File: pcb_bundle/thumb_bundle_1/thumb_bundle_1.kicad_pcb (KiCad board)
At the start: 2 copper layers, 100.6 x 101.6 mm, 55 parts

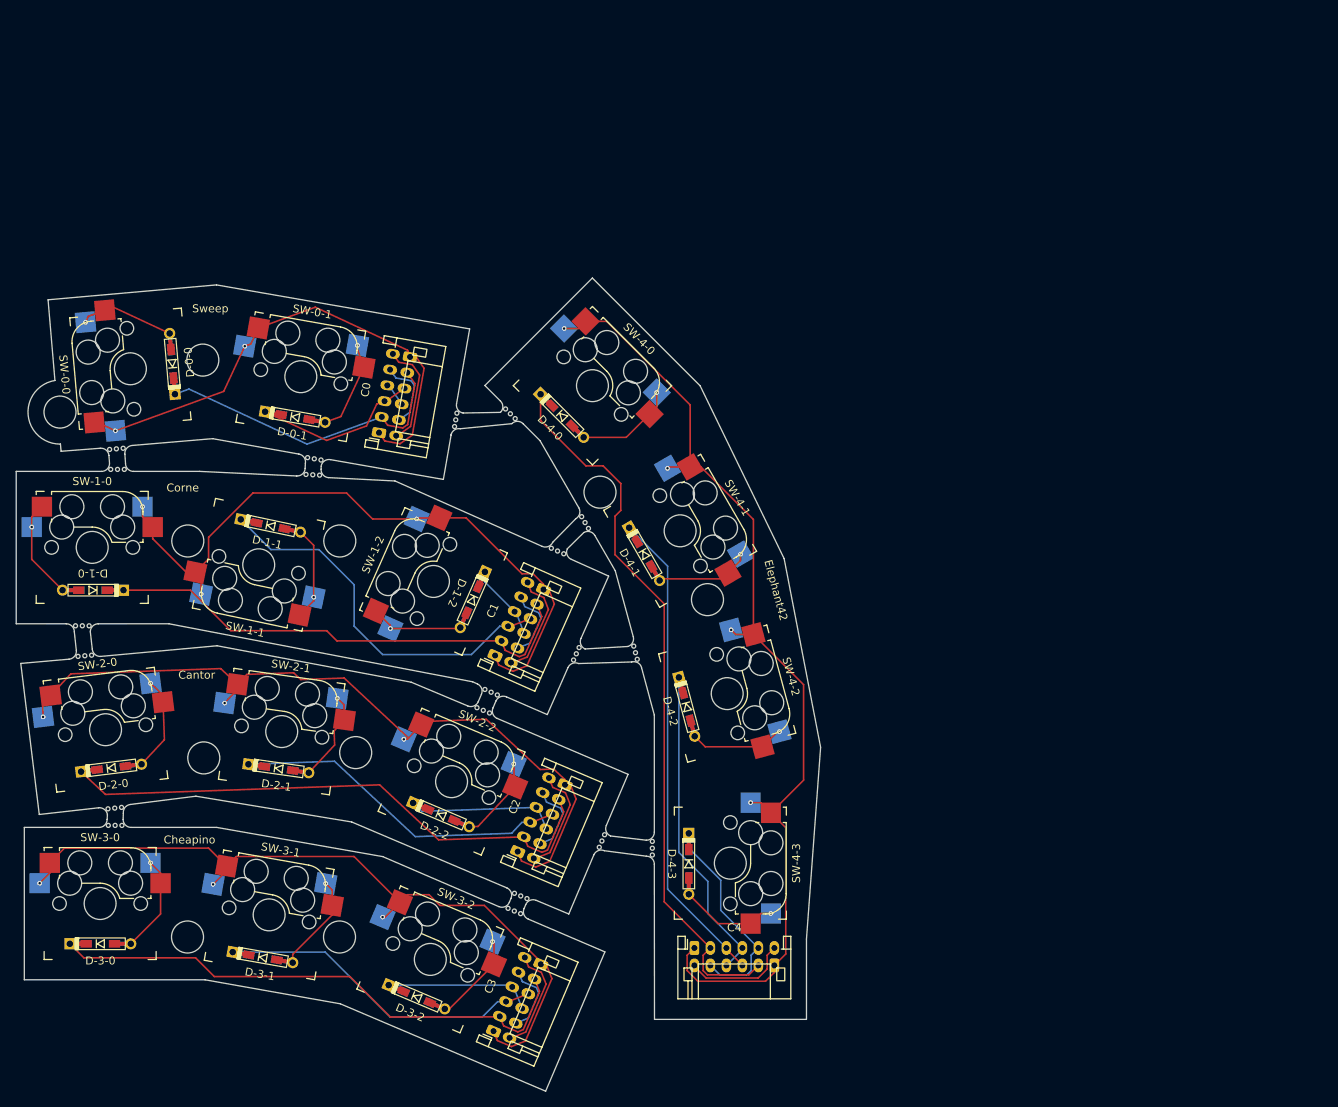
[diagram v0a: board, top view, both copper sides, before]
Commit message: [unstable] interim state
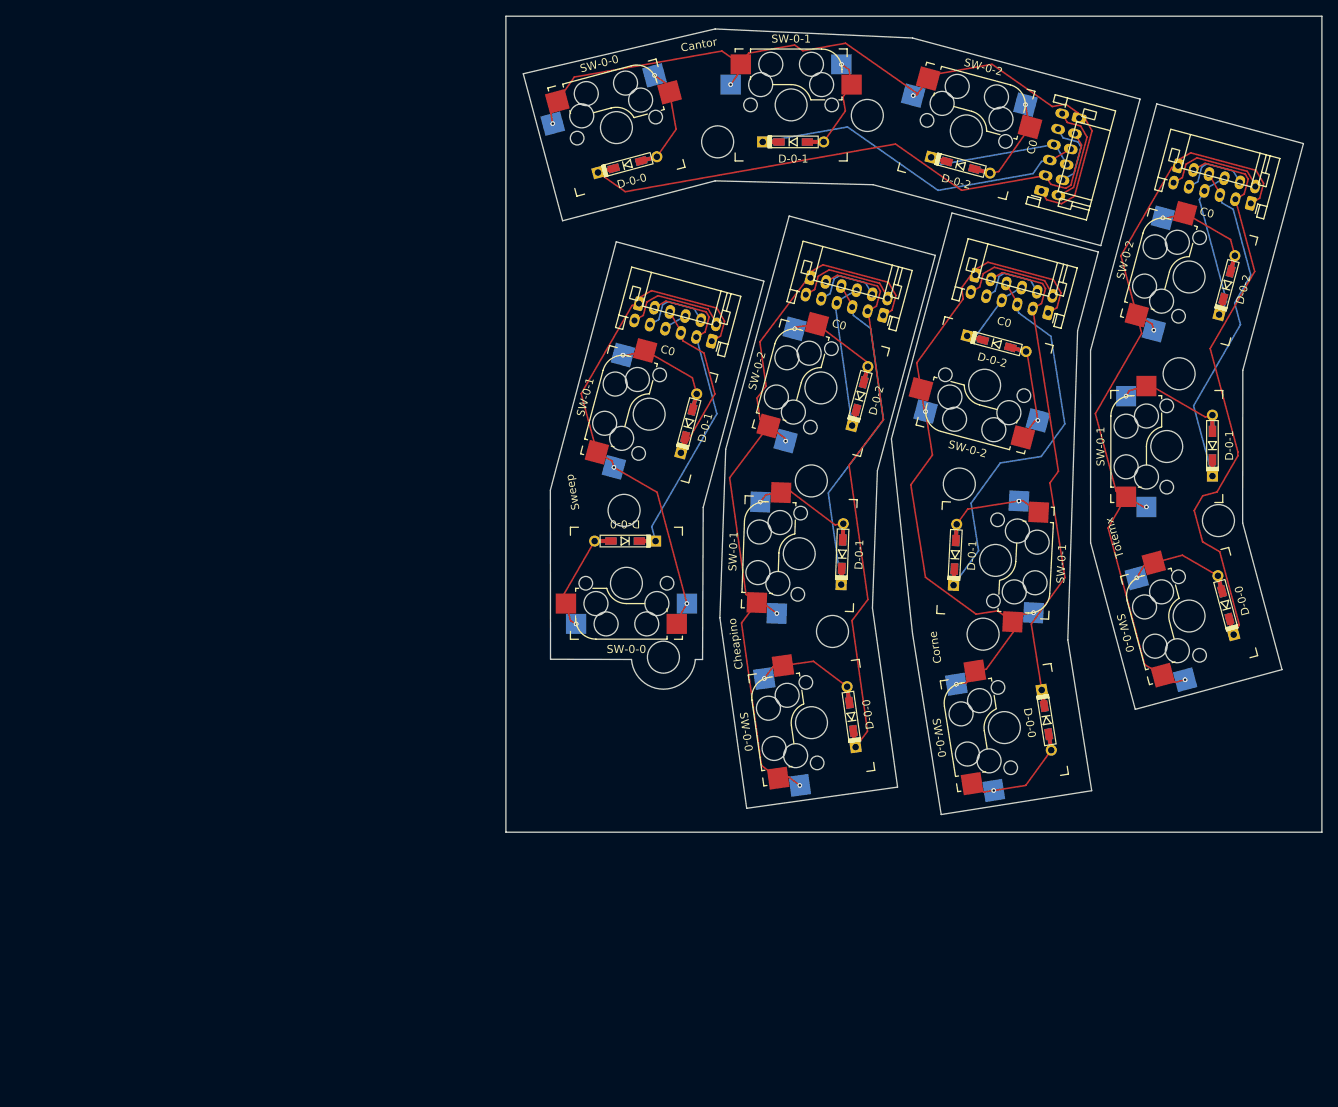
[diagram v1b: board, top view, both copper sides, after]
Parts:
- removed the C0 at (88.3, 65.3)
- removed C1, C2, C3, C4: Conn_01x06_Socket, crustrusk:reversible JST_PH_S6B-PH-K_1x06_P2.00mm_Horizontal
- removed the D-0-0 at (62.4, 56.6)
- removed the D-0-1 at (77.8, 63.3)
- removed D-1-0, D-1-1, D-1-2, D-2-0, D-2-1, D-2-2, D-3-0, D-3-1, D-3-2, D-4-0, D-4-1, D-4-2, D-4-3: D, crustrusk:Diode_TH_SMD_REVERSIBLE
- removed REF** (x20): MouseBite-Part_2.0x2.0mm_outset_D0.5mm_P0.85mm_3h, Panelization:MouseBite-Part_2.0x2.0mm_outset_D0.5mm_P0.85mm_3h
- removed the SW-0-0 at (57.2, 57.3)
- removed the SW-0-1 at (78.5, 58.3)
- removed SW-1-0, SW-1-1, SW-1-2, SW-2-0, SW-2-1, SW-2-2, SW-3-0, SW-3-1, SW-3-2, SW-4-0, SW-4-1, SW-4-2, SW-4-3: SW_Push, crustrusk:Kailh_hotswap_only_socket_MX_optional_reversible-MIRROR
- added C0: Conn_01x06_Socket, crustrusk:reversible JST_PH_S6B-PH-K_1x06_P2.00mm_Horizontal, F.Cu at (151.3, 50.6)
- added C0: Conn_01x06_Socket, crustrusk:reversible JST_PH_S6B-PH-K_1x06_P2.00mm_Horizontal, F.Cu at (129.9, 53.8)
- added C0: Conn_01x06_Socket, crustrusk:reversible JST_PH_S6B-PH-K_1x06_P2.00mm_Horizontal, F.Cu at (197.3, 36.6)
- added C0: Conn_01x06_Socket, crustrusk:reversible JST_PH_S6B-PH-K_1x06_P2.00mm_Horizontal, F.Cu at (171.1, 35.0)
- added C0: Conn_01x06_Socket, crustrusk:reversible JST_PH_S6B-PH-K_1x06_P2.00mm_Horizontal, F.Cu at (171.9, 50.3)
- added D-0-0: D, crustrusk:Diode_TH_SMD_REVERSIBLE, F.Cu at (119.0, 78.8)
- added D-0-0: D, crustrusk:Diode_TH_SMD_REVERSIBLE, F.Cu at (119.3, 31.8)
- added D-0-0: D, crustrusk:Diode_TH_SMD_REVERSIBLE, F.Cu at (147.3, 100.8)
- added D-0-0: D, crustrusk:Diode_TH_SMD_REVERSIBLE, F.Cu at (171.7, 101.2)
- added D-0-0: D, crustrusk:Diode_TH_SMD_REVERSIBLE, F.Cu at (194.1, 86.8)
- added D-0-1: D, crustrusk:Diode_TH_SMD_REVERSIBLE, F.Cu at (127.0, 64.1)
- added D-0-1: D, crustrusk:Diode_TH_SMD_REVERSIBLE, F.Cu at (192.5, 66.9)
- added D-0-1: D, crustrusk:Diode_TH_SMD_REVERSIBLE, F.Cu at (146.2, 80.4)
- added D-0-1: D, crustrusk:Diode_TH_SMD_REVERSIBLE, F.Cu at (140.1, 28.9)
- added D-0-1: D, crustrusk:Diode_TH_SMD_REVERSIBLE, F.Cu at (160.3, 80.5)
- added D-0-2: D, crustrusk:Diode_TH_SMD_REVERSIBLE, F.Cu at (161.0, 31.8)
- added D-0-2: D, crustrusk:Diode_TH_SMD_REVERSIBLE, F.Cu at (194.3, 46.8)
- added D-0-2: D, crustrusk:Diode_TH_SMD_REVERSIBLE, F.Cu at (165.5, 54.1)
- added D-0-2: D, crustrusk:Diode_TH_SMD_REVERSIBLE, F.Cu at (148.4, 60.7)
- added SW-0-0: SW_Push, crustrusk:Kailh_hotswap_only_socket_MX_optional_reversible-MIRROR, F.Cu at (142.3, 101.5)
- added SW-0-0: SW_Push, crustrusk:Kailh_hotswap_only_socket_MX_optional_reversible-MIRROR, F.Cu at (118.0, 27.1)
- added SW-0-0: SW_Push, crustrusk:Kailh_hotswap_only_socket_MX_optional_reversible-MIRROR, F.Cu at (189.5, 88.2)
- added SW-0-0: SW_Push, crustrusk:Kailh_hotswap_only_socket_MX_optional_reversible-MIRROR, F.Cu at (119.2, 84.1)
- added SW-0-0: SW_Push, crustrusk:Kailh_hotswap_only_socket_MX_optional_reversible-MIRROR, B.Cu at (166.5, 102.1)
- added SW-0-1: SW_Push, crustrusk:Kailh_hotswap_only_socket_MX_optional_reversible-MIRROR, F.Cu at (140.8, 80.4)
- added SW-0-1: SW_Push, crustrusk:Kailh_hotswap_only_socket_MX_optional_reversible-MIRROR, F.Cu at (122.1, 62.9)
- added SW-0-1: SW_Push, crustrusk:Kailh_hotswap_only_socket_MX_optional_reversible-MIRROR, F.Cu at (139.8, 24.3)
- added SW-0-1: SW_Push, crustrusk:Kailh_hotswap_only_socket_MX_optional_reversible-MIRROR, F.Cu at (186.8, 67.0)
- added SW-0-1: SW_Push, crustrusk:Kailh_hotswap_only_socket_MX_optional_reversible-MIRROR, B.Cu at (165.3, 81.2)
- added SW-0-2: SW_Push, crustrusk:Kailh_hotswap_only_socket_MX_optional_reversible-MIRROR, F.Cu at (161.7, 27.5)
- added SW-0-2: SW_Push, crustrusk:Kailh_hotswap_only_socket_MX_optional_reversible-MIRROR, F.Cu at (143.5, 59.7)
- added SW-0-2: SW_Push, crustrusk:Kailh_hotswap_only_socket_MX_optional_reversible-MIRROR, F.Cu at (189.5, 45.8)
- added SW-0-2: SW_Push, crustrusk:Kailh_hotswap_only_socket_MX_optional_reversible-MIRROR, B.Cu at (164.0, 59.3)
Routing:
- net COL0: track 63.7 -> 437.8 mm, vias 2 -> 14
- net ROW0-0: track 38.9 -> 309.7 mm
- net ROW1-0: track 20.7 -> 193.5 mm
- net COL4: track 125.2 -> 0.00 mm, vias 4 -> 0
- net COL2: track 97.3 -> 0.00 mm, vias 3 -> 0
- net COL3: track 95.1 -> 0.00 mm, vias 3 -> 0
- net ROW0-4: track 90.7 -> 0.00 mm
- net COL1: track 85.3 -> 0.00 mm, vias 3 -> 0
- net ROW0-2: track 70.0 -> 0.00 mm
- net ROW0-3: track 68.4 -> 0.00 mm
- net ROW2-0: track 2.83 -> 68.4 mm
- net ROW0-1: track 60.7 -> 0.00 mm
- net ROW1-4: track 60.4 -> 0.00 mm
- net ROW4-0: track 13.2 -> 65.9 mm
- net Net-(D-0-0-A): track 11.9 -> 60.5 mm, vias 1 -> 5
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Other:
- board size 100.6 x 101.6 mm -> 102 x 102 mm
- board text added: "Totemx"
- board text removed: "Elephant42"
